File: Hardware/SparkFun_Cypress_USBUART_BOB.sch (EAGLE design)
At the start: 41 parts, among them J1 MICROB, J3 FTDI_BASICPTH, U1 CY7C65213, U2 3.3V

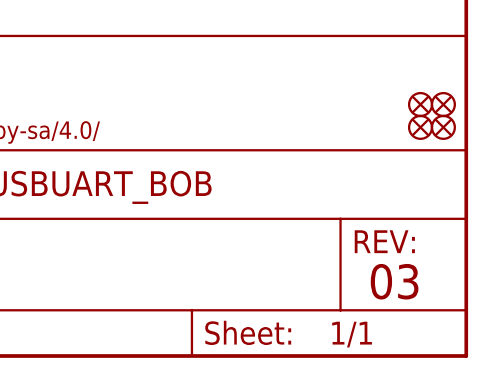
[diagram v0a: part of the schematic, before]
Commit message: Changed version number for reds
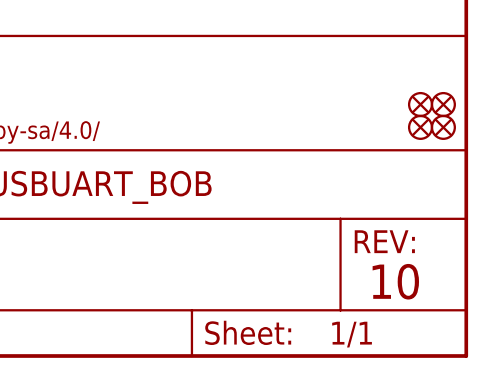
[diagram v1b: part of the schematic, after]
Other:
- note added: "10"
- note removed: "03"
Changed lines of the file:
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@@
 <?xml version="1.0" encoding="utf-8"?>
 <!DOCTYPE eagle SYSTEM "eagle.dtd">
-<eagle version="7.5.0">
+<eagle version="7.6.0">
 <drawing>
 <settings>
@@
 <layer number="255" name="routoute" color="7" fill="1" visible="yes" active="yes"/>
 </layers>
-<schematic xreflabel="%F%N/%S" xrefpart="/%S.%C%R">
+<schematic xreflabel="%F%N/%S" xrefpart="1_/%S.%C%R">
 <attributes>
 </attributes>
@@
 <sheet>
 <plain>
-<text x="237.998" y="6.35" size="3.81" layer="94" font="vector">03</text>
+<text x="237.998" y="6.35" size="3.81" layer="94" font="vector">10</text>
 <text x="154.432" y="6.096" size="3.81" layer="94" font="vector">Mike Hord</text>
 <text x="27.94" y="95.25" size="1.27" layer="97" font="vector">Open JP1 if VIO used

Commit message: Revert to v02.
Revert "Changed version number for reds"

This reverts commit 640f5162c93cb70f6f1d384f505e534c75df1209.
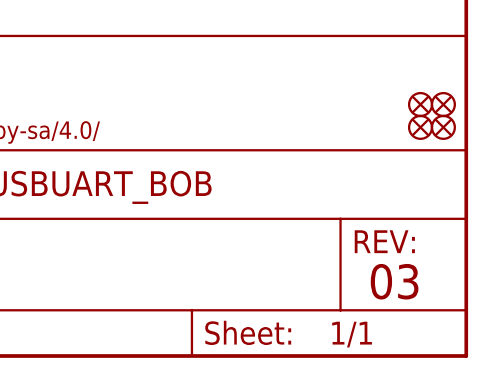
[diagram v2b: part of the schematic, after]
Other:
- note added: "03"
- note removed: "10"
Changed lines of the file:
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@@
 <?xml version="1.0" encoding="utf-8"?>
 <!DOCTYPE eagle SYSTEM "eagle.dtd">
-<eagle version="7.6.0">
+<eagle version="7.5.0">
 <drawing>
 <settings>
@@
 <layer number="255" name="routoute" color="7" fill="1" visible="yes" active="yes"/>
 </layers>
-<schematic xreflabel="%F%N/%S" xrefpart="1_/%S.%C%R">
+<schematic xreflabel="%F%N/%S" xrefpart="/%S.%C%R">
 <attributes>
 </attributes>
@@
 <sheet>
 <plain>
-<text x="237.998" y="6.35" size="3.81" layer="94" font="vector">10</text>
+<text x="237.998" y="6.35" size="3.81" layer="94" font="vector">03</text>
 <text x="154.432" y="6.096" size="3.81" layer="94" font="vector">Mike Hord</text>
 <text x="27.94" y="95.25" size="1.27" layer="97" font="vector">Open JP1 if VIO used

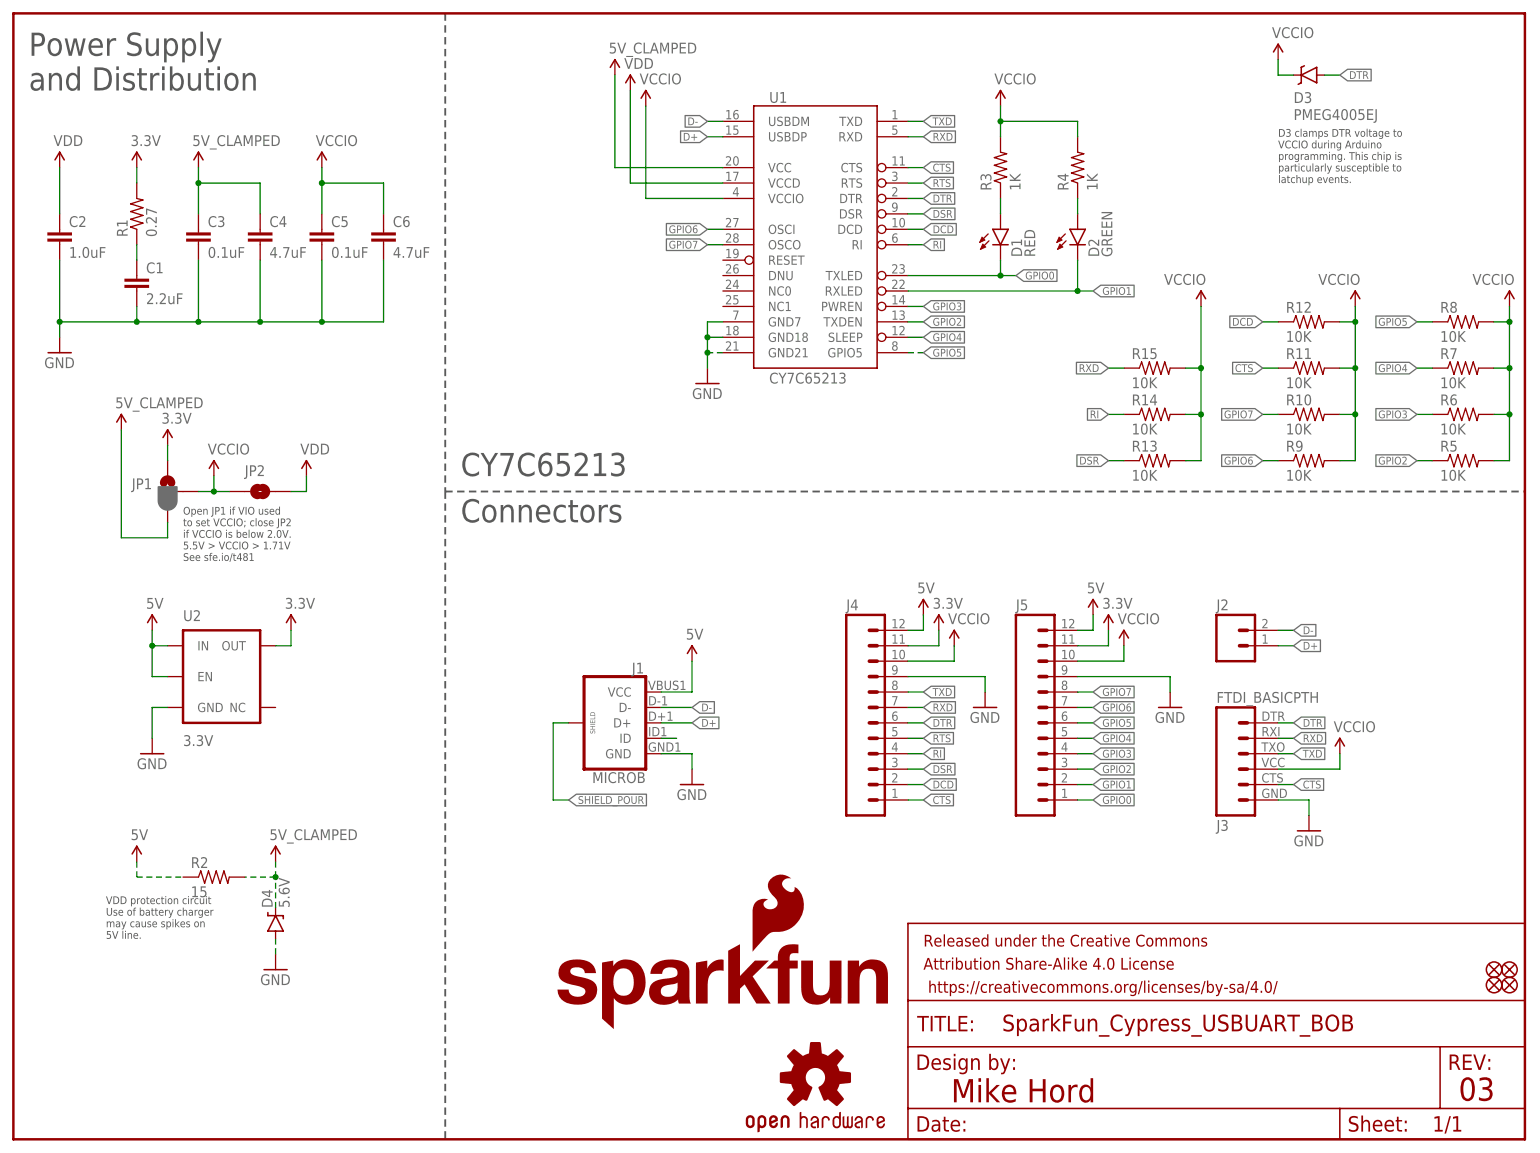
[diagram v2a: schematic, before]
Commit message: Revert to v02
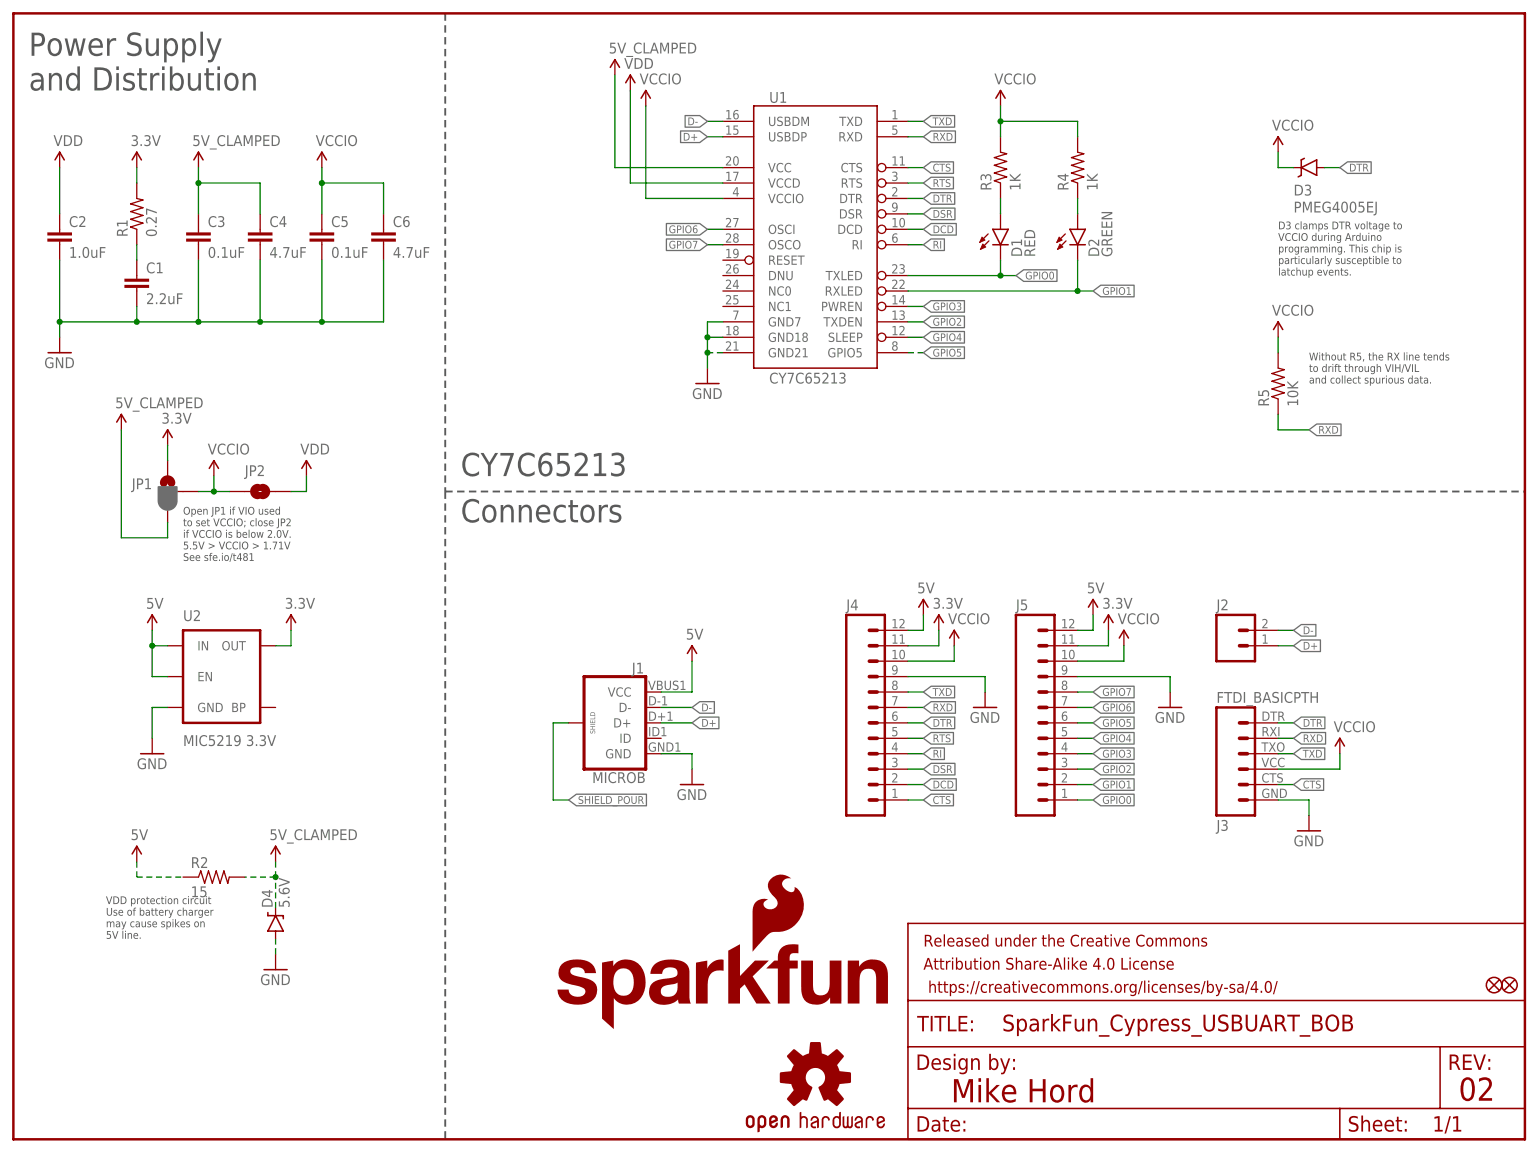
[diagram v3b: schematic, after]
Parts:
- removed FD3, FD4: FIDUCIALUFIDUCIAL, SparkFun-Aesthetics:FIDUCIALUFIDUCIAL
- removed R10, R11, R12, R13, R14, R15, R6, R7, R8, R9: 10K, SparkFun-Resistors:10KOHM-1/10W-1%(0603)0603
- U2: value 3.3V -> MIC5219 3.3V; device SparkFun-PowerIC:V_REG_AP2112K-3.3V -> SparkFun-PowerIC:V_REG_MIC52193.3V
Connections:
- removed net N$4: J1.ID
- net CTS: no longer R11.1
- net DCD: no longer R12.1
- net DSR: no longer R13.1
- net GPIO2: no longer R5.1
- net GPIO3: no longer R6.1
- net GPIO4: no longer R7.1
- net GPIO5: no longer R8.1
- net GPIO6: no longer R9.1
- net GPIO7: no longer R10.1
- net RI: no longer R14.1
- net RXD: now also R5.1; no longer R15.1
- net VCCIO: no longer R10.2, R11.2, R12.2, R13.2, R14.2, R15.2, R6.2, R7.2, R8.2, R9.2
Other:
- note added: "02"
- note added: "Without R5, the RX line tends to drift through VIH/VIL and collect spurious data."
- note removed: "03"
- moved on the sheet: D3, R5

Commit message: Changes from review incorporated
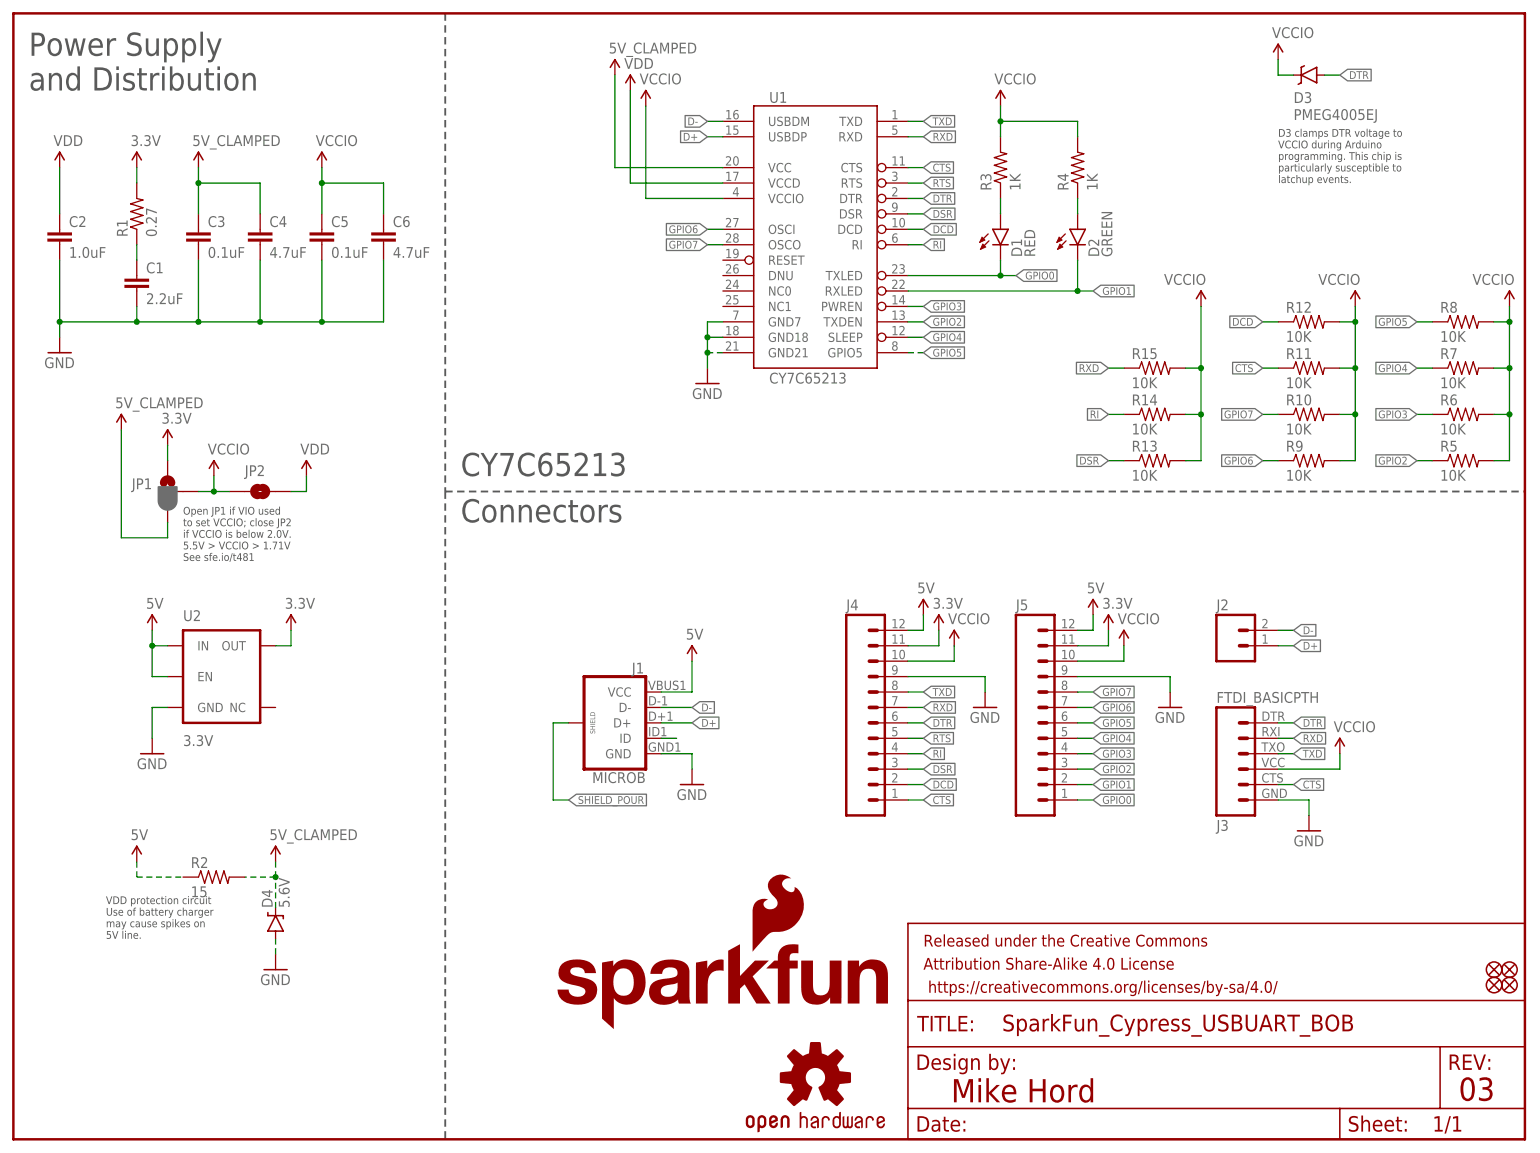
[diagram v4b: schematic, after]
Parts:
- added FD3, FD4: FIDUCIALUFIDUCIAL, SparkFun-Aesthetics:FIDUCIALUFIDUCIAL
- added R10, R11, R12, R13, R14, R15, R6, R7, R8, R9: 10K, SparkFun-Resistors:10KOHM-1/10W-1%(0603)0603
- U2: value MIC5219 3.3V -> 3.3V; device SparkFun-PowerIC:V_REG_MIC52193.3V -> SparkFun-PowerIC:V_REG_AP2112K-3.3V
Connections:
- new net N$4: J1.ID
- net CTS: now also R11.1
- net DCD: now also R12.1
- net DSR: now also R13.1
- net GPIO2: now also R5.1
- net GPIO3: now also R6.1
- net GPIO4: now also R7.1
- net GPIO5: now also R8.1
- net GPIO6: now also R9.1
- net GPIO7: now also R10.1
- net RI: now also R14.1
- net RXD: now also R15.1; no longer R5.1
- net VCCIO: now also R10.2, R11.2, R12.2, R13.2, R14.2, R15.2, R6.2, R7.2, R8.2, R9.2
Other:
- note added: "03"
- note removed: "02"
- note removed: "Without R5, the RX line tends to drift through VIH/VIL and collect spurious data."
- moved on the sheet: D3, R5
